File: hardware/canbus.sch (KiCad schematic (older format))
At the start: 14 parts, among them U2 MCP2515-xSO, U3 TJA1051T-3, Y1 8MHz

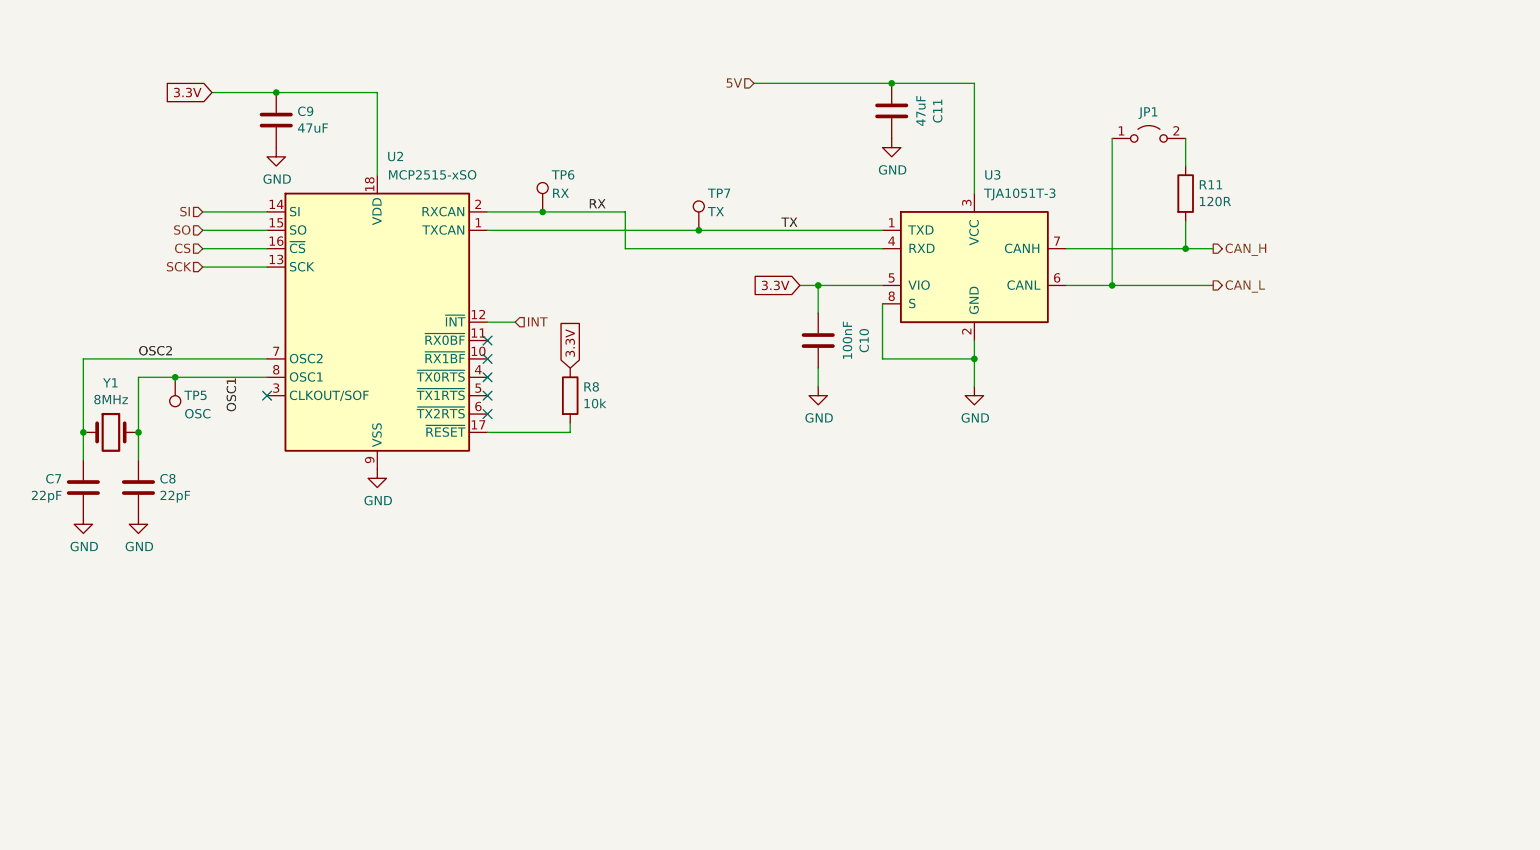
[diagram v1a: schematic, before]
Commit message: revE ready for production
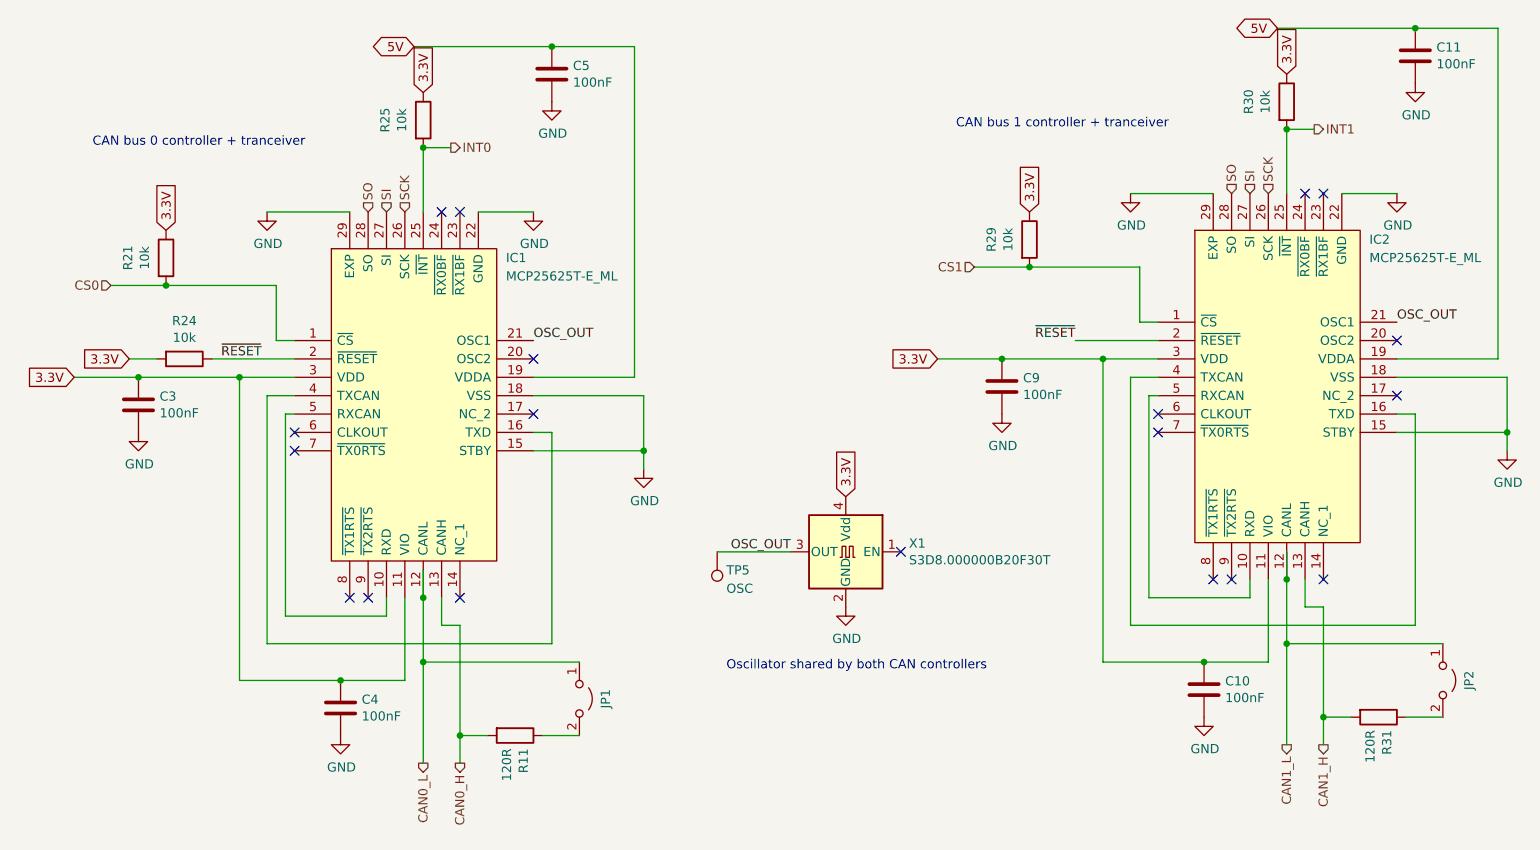
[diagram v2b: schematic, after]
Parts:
- removed C7, C8: 22pF, Capacitor_SMD:C_0603_1608Metric_Pad1.05x0.95mm_HandSolder, symbol Device:C
- removed R8: 10k, Resistor_SMD:R_0603_1608Metric_Pad1.05x0.95mm_HandSolder, symbol Device:R
- removed TP6: RX, TestPoint:TestPoint_Keystone_5000-5004_Miniature, symbol Connector:TestPoint
- removed TP7: TX, TestPoint:TestPoint_Keystone_5000-5004_Miniature, symbol Connector:TestPoint
- removed U2: MCP2515-xSO, Package_SO:SOIC-18W_7.5x11.6mm_P1.27mm, symbol pi-supercap-ups:MCP2515-xSO
- removed U3: TJA1051T-3, Package_SO:SOIC-8_3.9x4.9mm_P1.27mm, symbol pi-supercap-ups:TJA1051T-3
- removed Y1: 8MHz, Crystal:Crystal_HC49-U_Vertical, symbol Device:Crystal
- added C3, C4, C5: 100nF, Capacitor_SMD:C_0603_1608Metric_Pad1.05x0.95mm_HandSolder, symbol Device:C
- added IC1, IC2: MCP25625T-E_ML, custom:QFN65P600X600X100-29M-D, symbol pi-supercap-ups:MCP25625T-E_ML
- added JP2: Term, Connector_PinHeader_2.54mm:PinHeader_1x02_P2.54mm_Vertical, symbol Jumper:Jumper_2_Open
- added R21, R24, R25, R29, R30: 10k, Resistor_SMD:R_0603_1608Metric_Pad1.05x0.95mm_HandSolder, symbol Device:R
- added R31: 120R, Resistor_SMD:R_1206_3216Metric_Pad1.42x1.75mm_HandSolder, symbol Device:R
- added X1: S3D8.000000B20F30T, Oscillator:Oscillator_SMD_Abracon_ASE-4Pin_3.2x2.5mm, symbol Oscillator:ASE-xxxMHz
- C11, C9: value 47uF -> 100nF; footprint Capacitor_SMD:C_0805_2012Metric_Pad1.15x1.40mm_HandSolder -> Capacitor_SMD:C_0603_1608Metric_Pad1.05x0.95mm_HandSolder
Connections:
- net 3.3V: now also C10.1, C3.1, C4.1, IC1.11 (VIO), IC1.3 (VDD), IC2.11 (VIO), IC2.3 (VDD), R21.1, R24.2, R25.1, R29.1, R30.1, X1.4 (Vdd); no longer C10.2
- net 5V: now also C11.1, C5.1, IC1.19 (VDDA), IC2.19 (VDDA); no longer C11.2
- net GND: now also C10.2, C11.2, C3.2, C4.2, C5.2, IC1.15 (STBY), IC1.18 (VSS), IC1.22 (GND), IC1.29 (EXP), IC2.15 (STBY), IC2.18 (VSS), IC2.22 (GND), IC2.29 (EXP), X1.2 (GND); no longer C10.1, C11.1
- net SCK: now also IC1.26 (SCK), IC2.26 (SCK)
- net SI: now also IC1.27 (SI), IC2.27 (SI)
- net SO: now also IC1.28 (SO), IC2.28 (SO)
- net CAN_H renamed CAN0_H
- net CAN0_H: now also IC1.13 (CANH)
- net CAN_L renamed CAN0_L
- net CAN0_L: now also IC1.12 (CANL)
- net OSC1 renamed OSC_OUT
- net OSC_OUT: now also IC1.21 (OSC1), IC2.21 (OSC1), X1.3 (OUT)
- new net: IC1.10 (RXD), IC1.5 (RXCAN)
- new net: IC1.16 (TXD), IC1.4 (TXCAN)
- new net: IC2.10 (RXD), IC2.5 (RXCAN)
- new net: IC2.16 (TXD), IC2.4 (TXCAN)
- new net: JP2.2 (B), R31.1
- new net CAN1_H: IC2.13 (CANH), R31.2
- new net CAN1_L: IC2.12 (CANL), JP2.1 (A)
- new net CS0: IC1.1 (~CS), R21.2
- new net CS1: IC2.1 (~CS), R29.2
- new net INT0: IC1.25 (~INT), R25.2
- new net INT1: IC2.25 (~INT), R30.2
- new net ~RESET: IC1.2 (~RESET), IC2.2 (~RESET), R24.1
- no-connect marks 6 -> 19
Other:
- note added: "CAN bus 0 controller + tranceiver"
- note added: "CAN bus 1 controller + tranceiver"
- note added: "Oscillator shared by both CAN controllers"
- moved on the sheet: JP1, R11, TP5
